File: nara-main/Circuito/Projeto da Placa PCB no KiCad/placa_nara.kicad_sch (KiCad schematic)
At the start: 8 parts, among them J1 JETSON, J2 Motor Right, J3 Motor Left, J4 Encoder Right, J5 Encoder Left, U2 module_mpu6050, U3 LLC Encoders

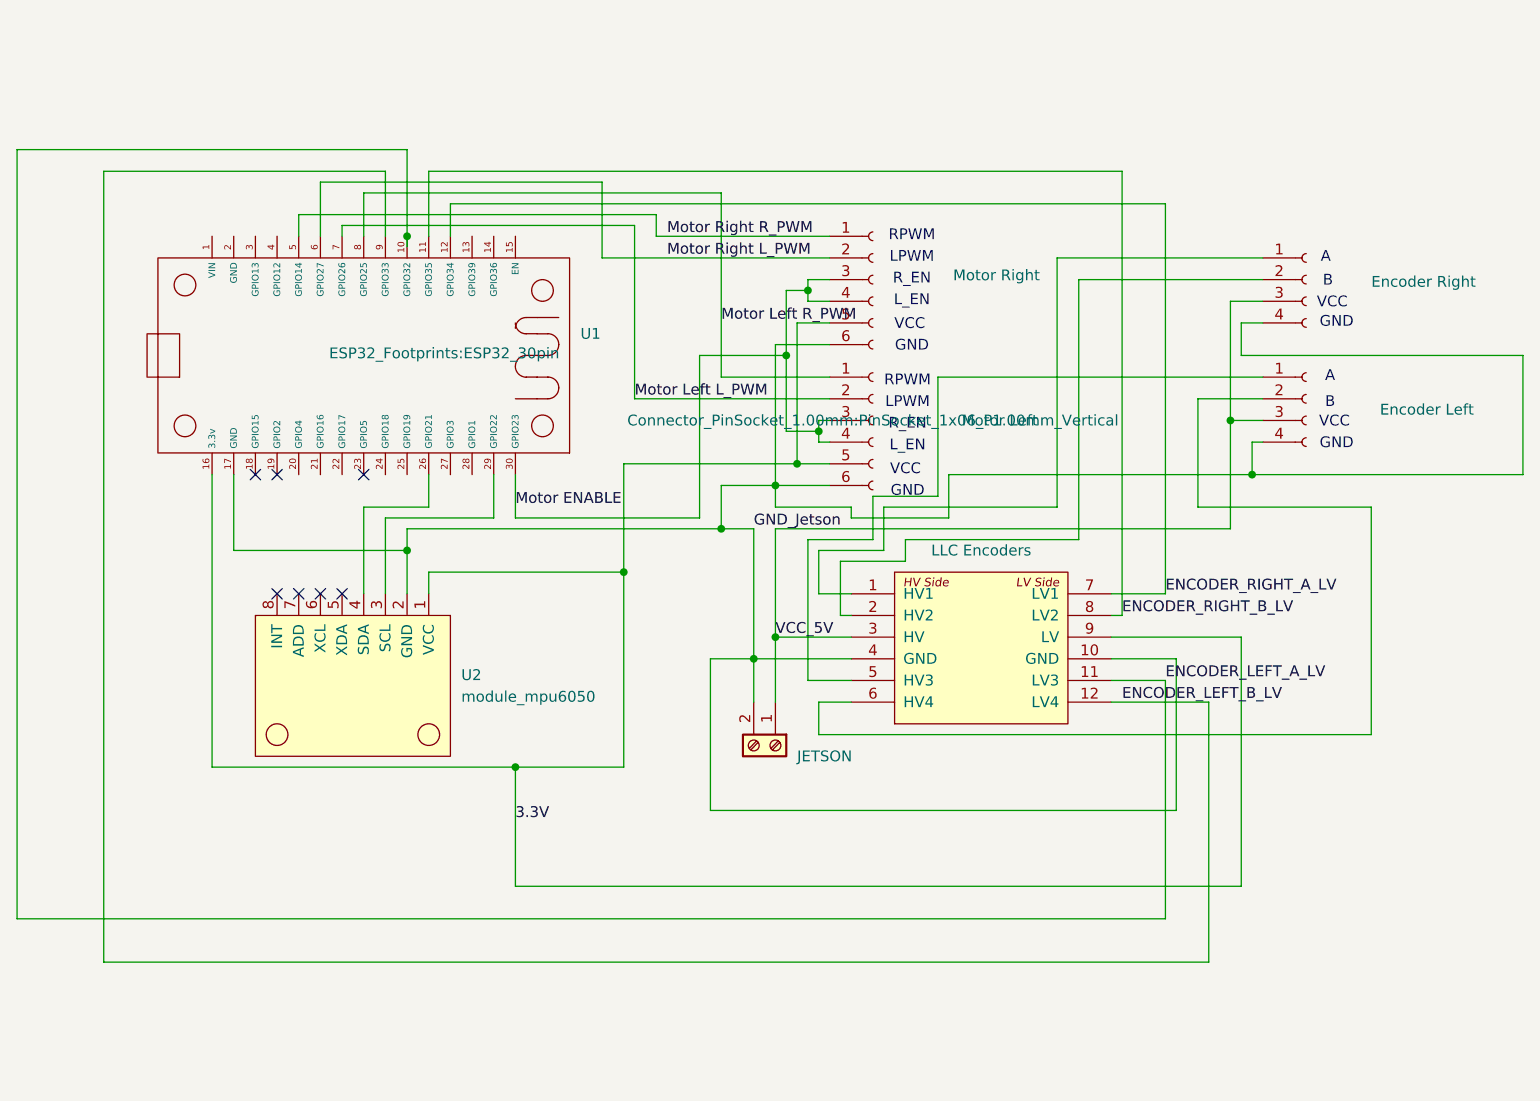
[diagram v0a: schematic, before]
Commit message: Projeto da Placa PCB Atualizado
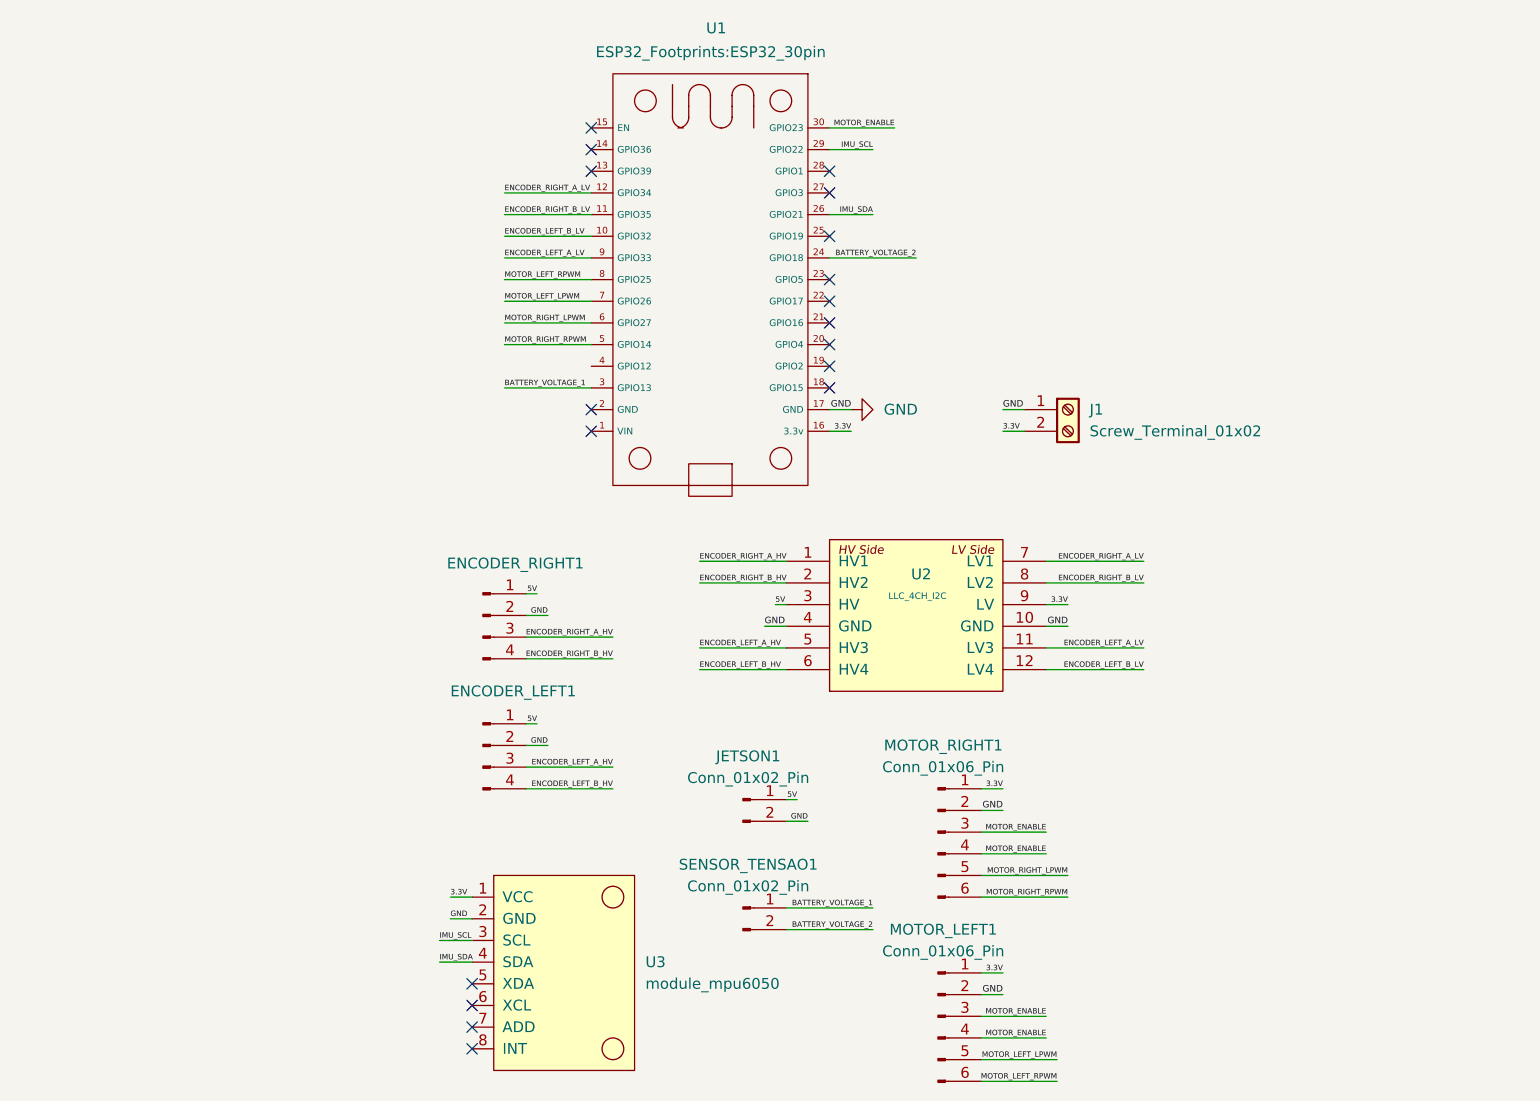
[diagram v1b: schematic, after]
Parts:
- removed J2: Motor Right, Connector_PinSocket_1.00mm:PinSocket_1x06_P1.00mm_Vertical, symbol Connector:Conn_01x06_Socket
- removed J3: Motor Left, Connector_PinSocket_1.00mm:PinSocket_1x06_P1.00mm_Vertical, symbol Connector:Conn_01x06_Socket
- removed J4: Encoder Right, Connector_PinSocket_1.00mm:PinSocket_1x04_P1.00mm_Vertical, symbol Connector:Conn_01x04_Socket
- removed J5: Encoder Left, Connector_PinSocket_1.00mm:PinSocket_1x04_P1.00mm_Vertical, symbol Connector:Conn_01x04_Socket
- removed U2: module_mpu6050, usini_sensors:module_mpu6050, symbol usini_sensors:module_mpu6050
- removed U3: LLC Encoders, LLC_4CH_I2C:LLC_4CH_I2C_MODULE, symbol LLC_4CH_I2C:LLC_4CH_I2C
- added ENCODER_LEFT1, ENCODER_RIGHT1: Conn_01x04_Pin, Connector_PinHeader_2.54mm:PinHeader_1x04_P2.54mm_Vertical, symbol Connector:Conn_01x04_Pin
- added JETSON1, SENSOR_TENSAO1: Conn_01x02_Pin, Connector_PinHeader_2.54mm:PinHeader_1x02_P2.54mm_Vertical, symbol Connector:Conn_01x02_Pin
- added MOTOR_LEFT1, MOTOR_RIGHT1: Conn_01x06_Pin, Connector_PinHeader_2.54mm:PinHeader_1x06_P2.54mm_Vertical, symbol Connector:Conn_01x06_Pin
- added U2: LLC_4CH_I2C, LLC_4CH_I2C:LLC_4CH_I2C_MODULE, symbol LLC_4CH_I2C:LLC_4CH_I2C
- added U3: module_mpu6050, usini_sensors:module_mpu6050, symbol usini_sensors:module_mpu6050
- J1: value JETSON -> Screw_Terminal_01x02; footprint TerminalBlock_Phoenix:TerminalBlock_Phoenix_MKDS-1,5-2_1x02_P5.00mm_Horizontal -> TerminalBlock_Phoenix:TerminalBlock_Phoenix_MKDS-1,5-2-5.08_1x02_P5.08mm_Horizontal
- U1: value ~ -> (none)
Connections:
- net VCC_5V is gone; now on net GND: J1.1 (Pin_1)
- net 3.3V: now also J1.2 (Pin_2), MOTOR_LEFT1.1 (Pin_1), MOTOR_RIGHT1.1 (Pin_1), U2.9 (LV), U3.1 (VCC)
- net ENCODER_LEFT_A_LV: now also U1.9 (GPIO33), U2.11 (LV3); no longer U1.10 (GPIO32)
- net ENCODER_LEFT_B_LV: now also U1.10 (GPIO32), U2.12 (LV4); no longer U1.9 (GPIO33)
- net ENCODER_RIGHT_A_LV: now also U2.7 (LV1)
- net ENCODER_RIGHT_B_LV: now also U2.8 (LV2)
- net IMU_SCL: now reaches U1.29 (GPIO22)
- net IMU_SCL: now also U3.3 (SCL)
- net IMU_SDA: now reaches U1.26 (GPIO21)
- net IMU_SDA: now also U3.4 (SDA)
- net BATTERY_VOLTAGE_2: now reaches U1.24 (GPIO18)
- net BATTERY_VOLTAGE_2: now also SENSOR_TENSAO1.2 (Pin_2)
- net BATTERY_VOLTAGE_1: now reaches U1.3 (GPIO13)
- net BATTERY_VOLTAGE_1: now also SENSOR_TENSAO1.1 (Pin_1)
- net GND_Jetson renamed GND
- net GND: now also ENCODER_LEFT1.2 (Pin_2), ENCODER_RIGHT1.2 (Pin_2), JETSON1.2 (Pin_2), MOTOR_LEFT1.2 (Pin_2), MOTOR_RIGHT1.2 (Pin_2), U2.10 (GND), U2.4 (GND), U3.2 (GND); no longer J1.2 (Pin_2)
- net Motor ENABLE renamed MOTOR_ENABLE
- net MOTOR_ENABLE: now also MOTOR_LEFT1.3 (Pin_3), MOTOR_LEFT1.4 (Pin_4), MOTOR_RIGHT1.3 (Pin_3), MOTOR_RIGHT1.4 (Pin_4)
- net Motor Left L_PWM renamed MOTOR_LEFT_LPWM
- net MOTOR_LEFT_LPWM: now also MOTOR_LEFT1.5 (Pin_5)
- net Motor Left R_PWM renamed MOTOR_LEFT_RPWM
- net MOTOR_LEFT_RPWM: now also MOTOR_LEFT1.6 (Pin_6)
- net Motor Right L_PWM renamed MOTOR_RIGHT_LPWM
- net MOTOR_RIGHT_LPWM: now also MOTOR_RIGHT1.5 (Pin_5)
- net Motor Right R_PWM renamed MOTOR_RIGHT_RPWM
- net MOTOR_RIGHT_RPWM: now also MOTOR_RIGHT1.6 (Pin_6)
- new net 5V: ENCODER_LEFT1.1 (Pin_1), ENCODER_RIGHT1.1 (Pin_1), JETSON1.1 (Pin_1), U2.3 (HV)
- new net ENCODER_LEFT_A_HV: ENCODER_LEFT1.3 (Pin_3), U2.5 (HV3)
- new net ENCODER_LEFT_B_HV: ENCODER_LEFT1.4 (Pin_4), U2.6 (HV4)
- new net ENCODER_RIGHT_A_HV: ENCODER_RIGHT1.3 (Pin_3), U2.1 (HV1)
- new net ENCODER_RIGHT_B_HV: ENCODER_RIGHT1.4 (Pin_4), U2.2 (HV2)
- no-connect marks 7 -> 18
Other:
- note removed: "A"
- note removed: "B"
- note removed: "GND"
- note removed: "LPWM"
- note removed: "L_EN"
- note removed: "RPWM"
- note removed: "R_EN"
- note removed: "VCC"
